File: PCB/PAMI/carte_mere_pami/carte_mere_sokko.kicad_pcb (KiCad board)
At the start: 2 copper layers, 78.5 x 54 mm, 35 parts, among them IC1 ESP32-S3-WROOM-1-N16R8, IC2 LDO_3.3V_bis, J1 Conn_01x08_Socket, J10 Conn_01x07_Socket, J11 Conn_01x07_Socket, J12 Conn_Servos, J14 LiDAR Connector, J2 Connector 5V, J3 Connector 3.3V, J4 Micro_USB_pads_USB3075-30-A, J5 Conn_01x08_Socket, J6 Conn_01x04_Pin, J7 Conn_01x04_Pin, J8 Conn_01x08_Socket, J9 Conn_01x08_Socket, U1 ICM-45686

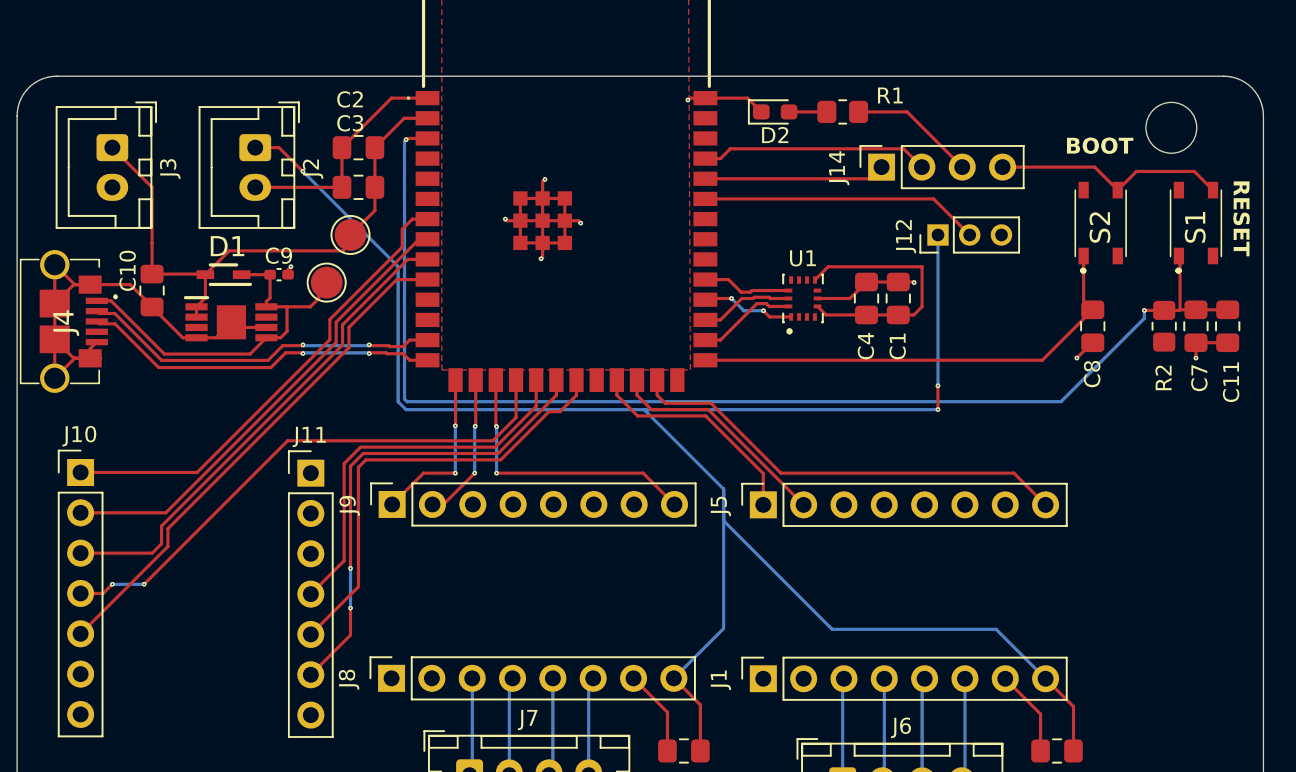
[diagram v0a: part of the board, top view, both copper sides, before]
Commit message: Fix PCB
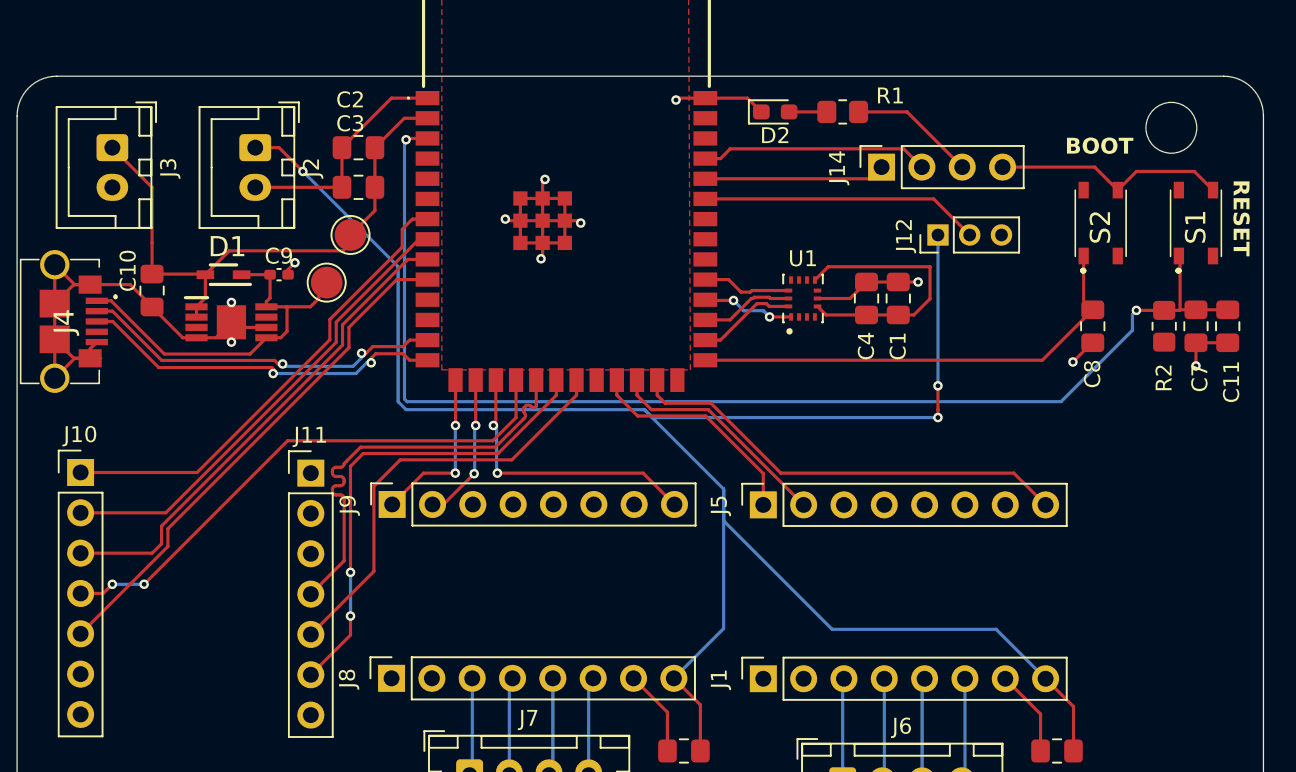
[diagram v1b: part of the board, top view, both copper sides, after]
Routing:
- net MOSI_LoRa: track 24.3 -> 27.0 mm
- net GND: track 111.8 -> 114.0 mm, vias 9 -> 11
- net MISO_LoRa: track 28.3 -> 27.1 mm
- net +3.3V: track 61.1 -> 61.8 mm
- net +5V: track 123.1 -> 123.8 mm
- net USB_D+: track 22.7 -> 23.2 mm
